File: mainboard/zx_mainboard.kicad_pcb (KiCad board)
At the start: 2 copper layers, 149.9 x 130.2 mm, 93 parts, among them P1 CONN_02X17, P2 CONN_02X20, P3 CONN_02X20, P4 CONN_01X02, P5 CONN_01X02, Q1 BSS123, Q2 BSS123, Q3 BSS123, Q4 BSS123, Q5 BSS123, Q6 BSS123, Q7 BSS123, Q8 BSS123, U1 4066, U2 4066, U3 4066, U4 4066, U5 4066, U6 74HC14, U7 74HC14

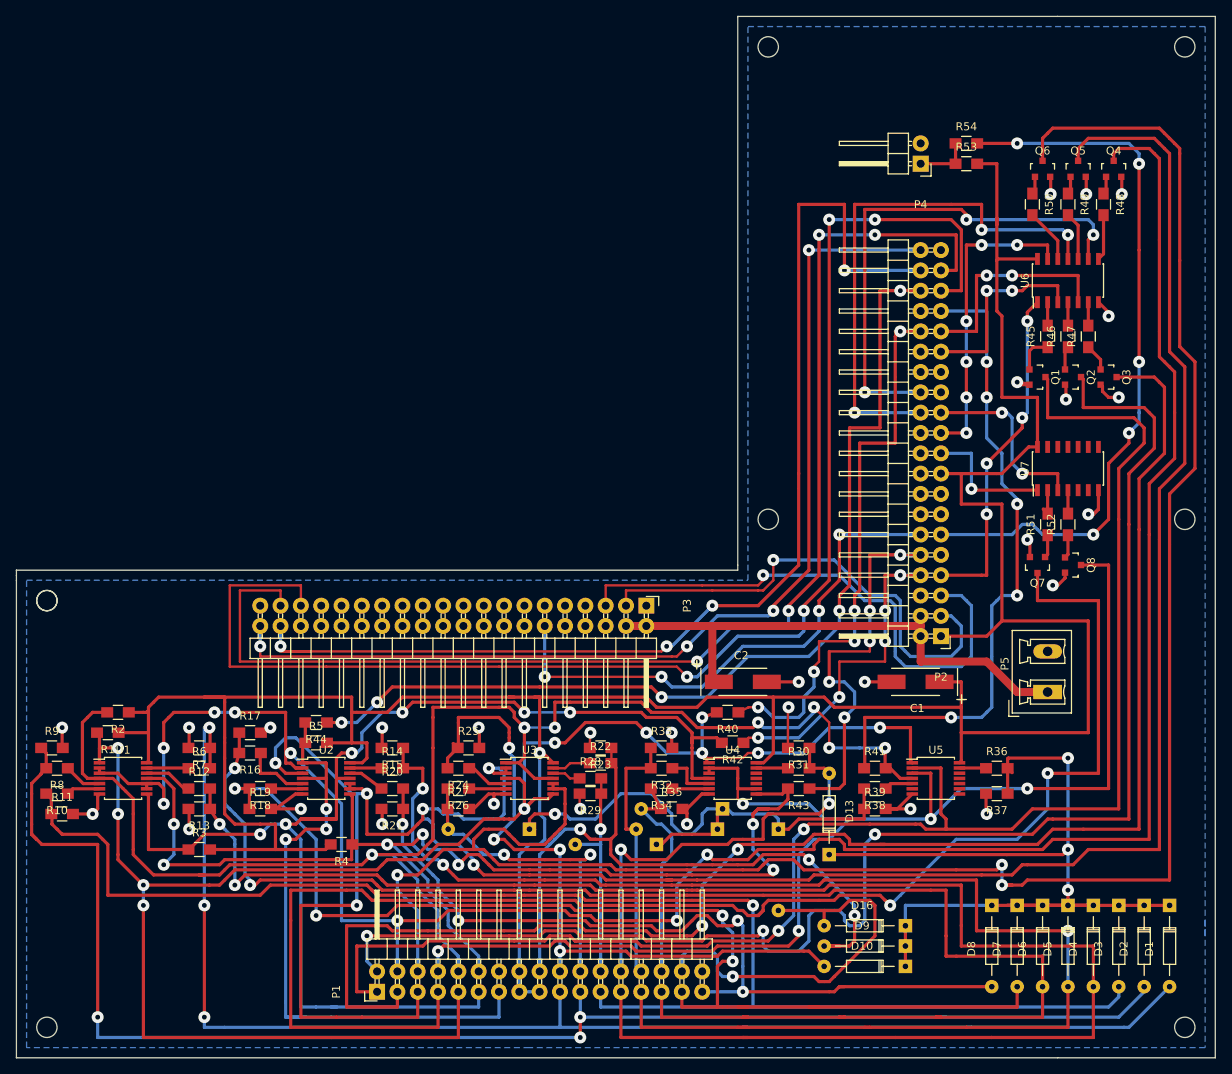
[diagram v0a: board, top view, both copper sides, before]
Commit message: pcb
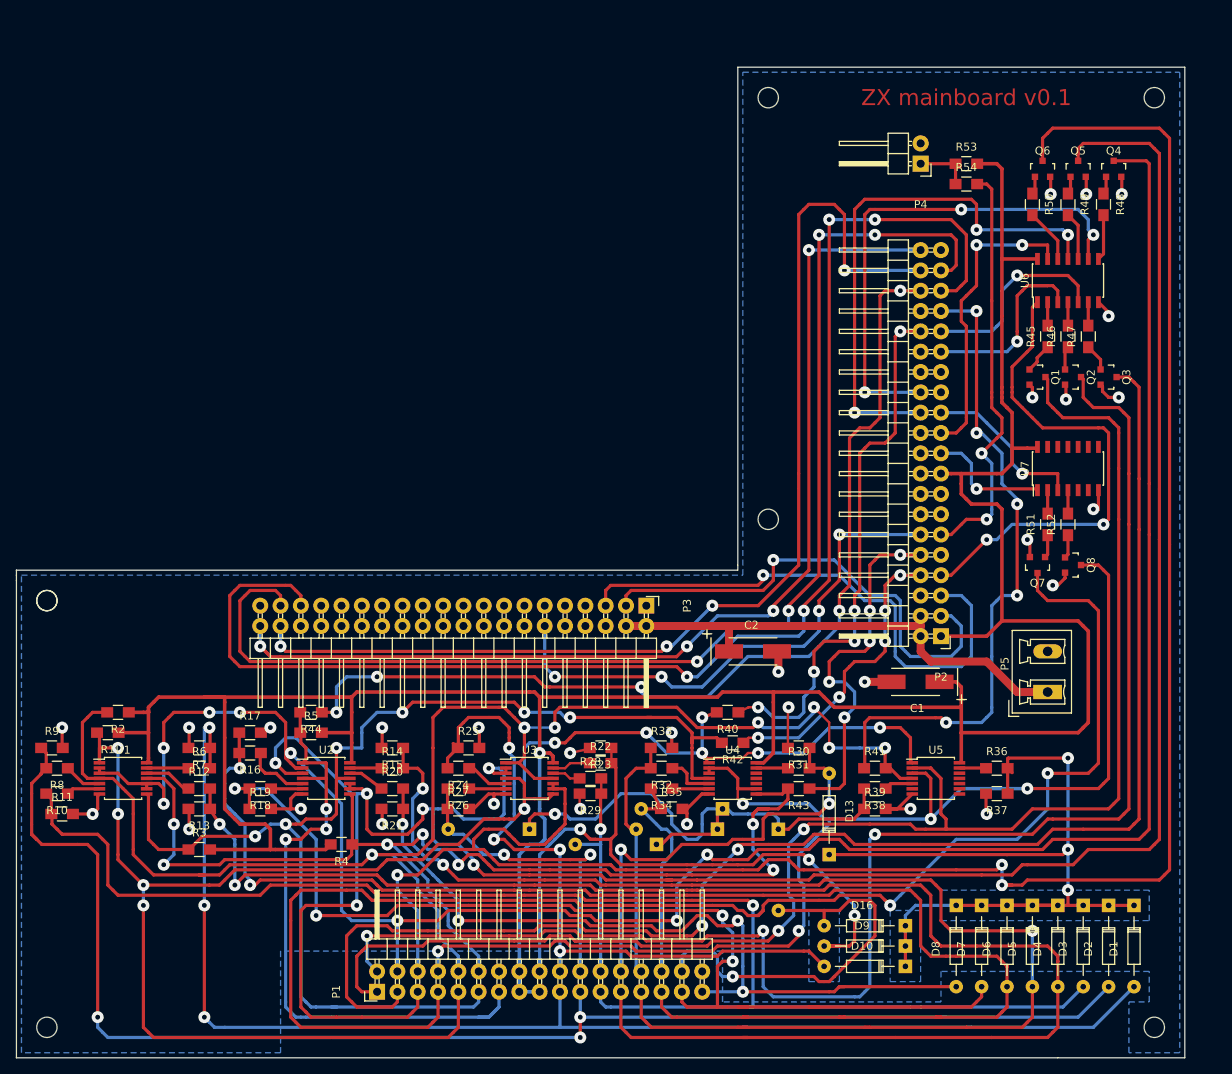
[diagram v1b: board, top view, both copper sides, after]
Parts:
- moved R54 5.08 mm to (161.3, 37.5)
- moved D5 4.45 mm to (169.5, 127.6)
- moved D1 4.44 mm to (182.2, 127.6)
- moved D2 4.44 mm to (179.1, 127.6)
- moved D3 4.44 mm to (175.9, 127.6)
- moved D4 4.44 mm to (172.7, 127.6)
- moved D6 4.44 mm to (166.4, 127.6)
- moved D7 4.44 mm to (163.2, 127.6)
- moved D8 4.44 mm to (160.0, 127.6)
- moved C2 4.02 mm to (134.6, 95.9)
- moved R44 1.42 mm to (79.4, 103.5)
- moved R5 1.42 mm to (79.4, 106.0)
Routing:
- net /GPIO16: track 199.1 -> 152.5 mm
- net +3V3: track 415.5 -> 369.2 mm
- net /GPIO12: track 123.1 -> 83.7 mm
- net /GPIO17: track 90.9 -> 52.2 mm, vias 5 -> 2
- net /GPIO20: track 184.6 -> 164.9 mm
- net /GPIO4: track 42.5 -> 61.8 mm, vias 4 -> 2
- net /CS_CTRL: track 125.1 -> 111.1 mm
- net /KIV: track 206.6 -> 194.0 mm
- net /KA10: track 197.0 -> 184.4 mm
- net /KLEFT: track 177.5 -> 165.2 mm
- net /KDOWN: track 190.0 -> 178.4 mm
- net /GPIO19: track 212.1 -> 201.1 mm
- net /GPIO6: track 34.4 -> 24.9 mm, vias 2 -> 1
- net /KD1: track 214.1 -> 204.8 mm
- net /GPIO26: track 214.5 -> 205.6 mm
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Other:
- board size 149.9 x 130.2 mm -> 146.1 x 123.8 mm
- net class 3.3v added: clearance 0.2, trace_width 0.45, via_dia 1.5, via_drill 0.6
- board text added: "ZX mainboard v0.1"
